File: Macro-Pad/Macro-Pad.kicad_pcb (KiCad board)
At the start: 2 copper layers, 42 x 80.5 mm, 14 parts, among them J1 USB_C_Receptacle_USB2.0_14P, U1 ESP32-S3-WROOM-1, U2 TPS62162DSG

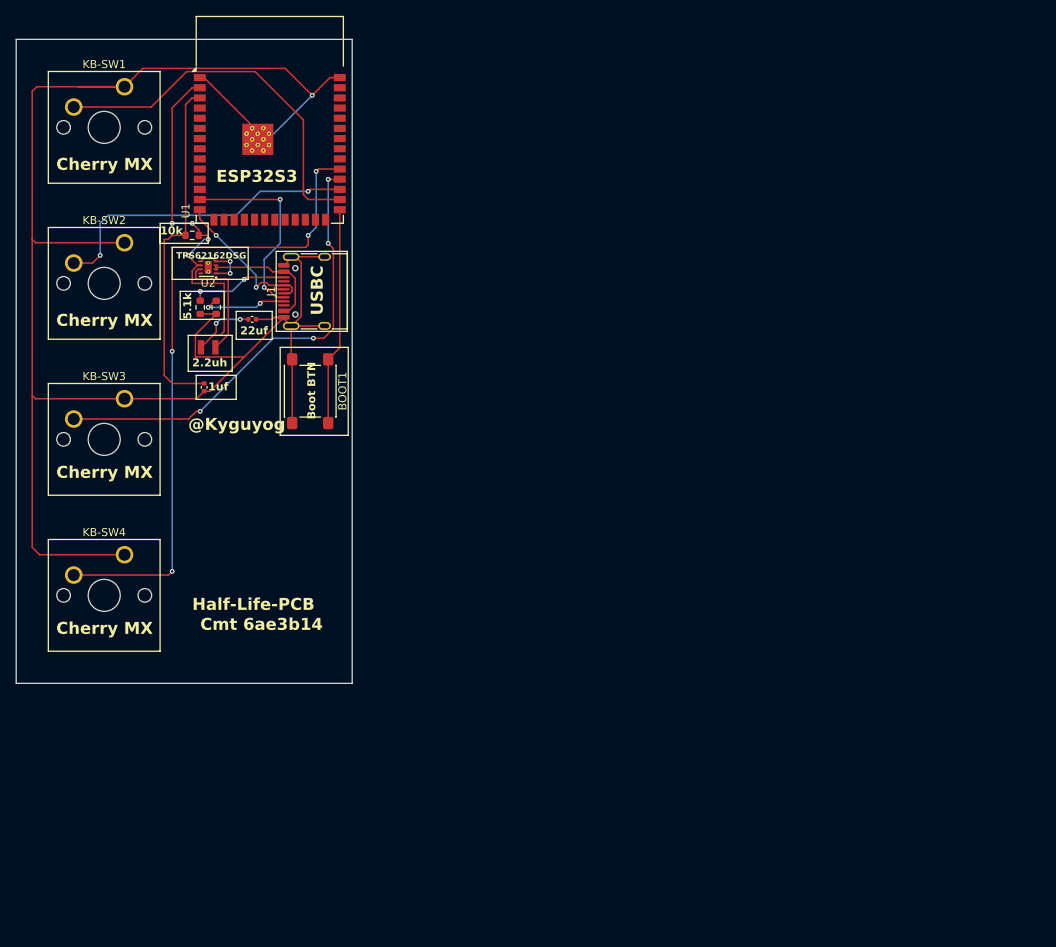
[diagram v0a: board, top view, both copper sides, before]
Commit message: re-format everything to save and optimize space
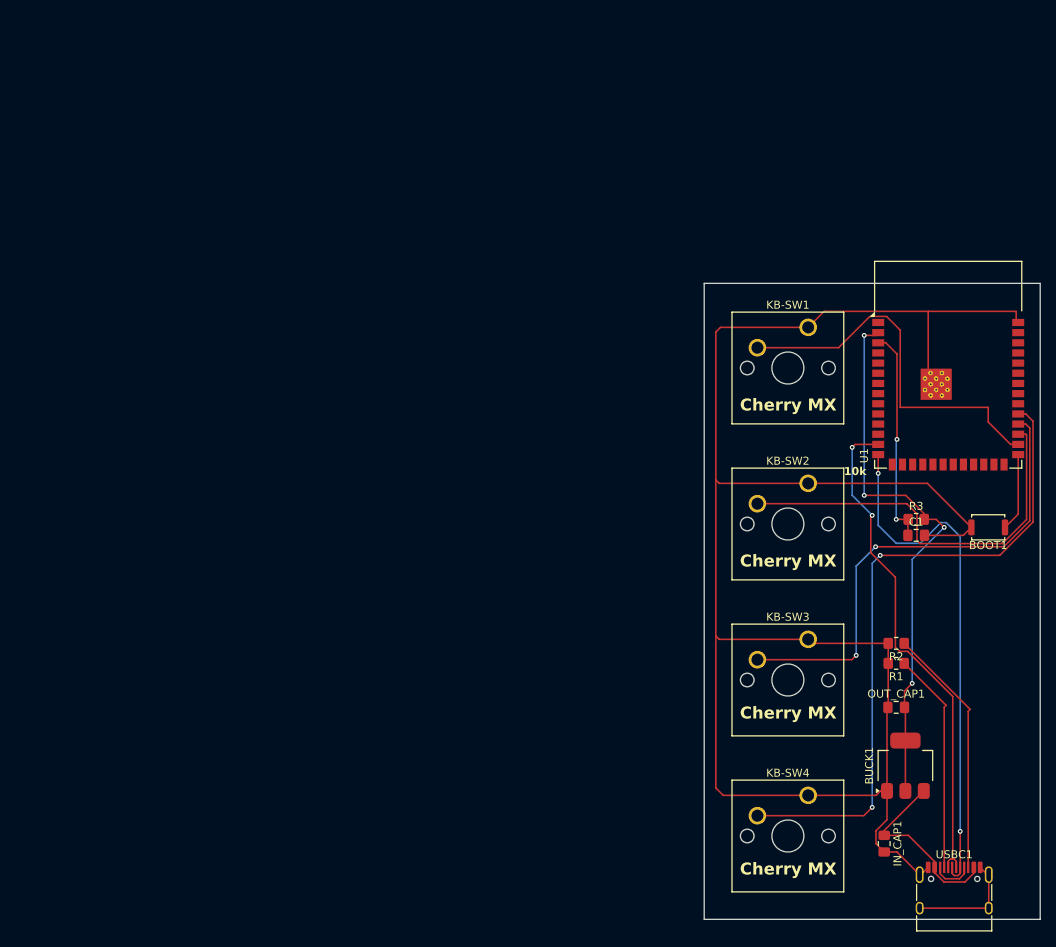
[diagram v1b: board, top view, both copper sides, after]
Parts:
- removed C2: 22uF, PCM_SparkFun-Capacitor:C_0402_1005Metric
- removed J1: USB_C_Receptacle_USB2.0_14P, Connector_USB:USB_C_Receptacle_HRO_TYPE-C-31-M-12
- removed L1: 2.2uH, PCM_SparkFun-Coil:0806
- removed U2: TPS62162DSG, Package_SON:Texas_DSG0008A_WSON-8-1EP_2x2mm_P0.5mm_EP0.9x1.6mm_ThermalVias
- added BUCK1: AMS1117-3.3, Package_TO_SOT_SMD:SOT-223-3_TabPin2, F.Cu at (124.2, 103.8)
- added IN_CAP1: 10uF, Capacitor_SMD:C_0805_2012Metric_Pad1.18x1.45mm_HandSolder, F.Cu at (121.5, 113.5)
- added OUT_CAP1: 22uF, Capacitor_SMD:C_0805_2012Metric_Pad1.18x1.45mm_HandSolder, F.Cu at (123.0, 96.5)
- added USBC1: USB_C_Receptacle_USB2.0_14P, Connector_USB:USB_C_Receptacle_HRO_TYPE-C-31-M-12, F.Cu at (130.2, 120.5)
- BOOT1: footprint Button_Switch_SMD:SW_SPST_PTS645Sx43SMTR92 -> Button_Switch_SMD:SW_Push_SPST_NO_Alps_SKRK
- C1: footprint PCM_SparkFun-Capacitor:C_0402_1005Metric -> Capacitor_SMD:C_0805_2012Metric_Pad1.18x1.45mm_HandSolder
- R1, R2, R3: footprint PCM_SparkFun-Resistor:R_0603_1608Metric -> Resistor_SMD:R_0805_2012Metric_Pad1.20x1.40mm_HandSolder
- moved R3 97.2 mm to (125.5, 73.0)
- moved R2 96.6 mm to (123.0, 88.5), turned to 180 degrees
- moved R1 95.9 mm to (123.0, 91.0), turned to 180 degrees
- moved C1 90.9 mm to (125.5, 75.0), turned to 0 degrees
- moved KB-SW1 90.6 mm to (112.0, 49.0)
- moved KB-SW2 90.6 mm to (112.0, 68.5)
- moved KB-SW3 90.6 mm to (112.0, 88.0)
- moved KB-SW4 90.6 mm to (112.0, 107.5)
- moved U1 90.2 mm to (129.5, 53.6)
- moved BOOT1 86.4 mm to (134.5, 74.0), turned to 180 degrees
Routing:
- net Net-(U1-USB_D+): track 19.2 -> 65.9 mm
- net Net-(U1-USB_D-): track 26.8 -> 63.6 mm
- net Net-(BUCK1-VI): track 0.00 -> 23.2 mm
- net Net-(USBC1-CC2): track 12.4 -> 31.5 mm, vias 2 -> 0
- net Net-(U1-IO0): track 27.3 -> 9.78 mm
- net Net-(USBC1-CC1): track 11.1 -> 27.8 mm, vias 2 -> 0
- net Net-(U1-EN): track 43.8 -> 27.3 mm, vias 0 -> 2
- net Net-(BUCK1-VO): track 52.5 -> 69.0 mm, vias 6 -> 4
- net Net-(U2-EN): track 16.1 -> 0.00 mm
- net Net-(U2-SW): track 14.9 -> 0.00 mm
- net Net-(U1-IO36): track 39.4 -> 50.6 mm, vias 2 -> 0
- net Net-(U2-AGND): track 7.29 -> 0.00 mm, vias 2 -> 0
- net (no net): track 0.00 -> 5.13 mm
- net Net-(BUCK1-GND): track 234.0 -> 238.9 mm, vias 1 -> 0
- net Net-(U1-IO37): track 57.5 -> 61.0 mm, vias 4 -> 2
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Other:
- board size 42 x 80.5 mm -> 42 x 79.5 mm
- board text removed: "1uf"
- board text removed: "2.2uh"
- board text removed: "22uf"
- board text removed: "5.1k"
- board text removed: "@Kyguyog"
- board text removed: "Boot BTN"
- board text removed: "Cmt 6ae3b14"
- board text removed: "ESP32S3"
- board text removed: "Half-Life-PCB"
- board text removed: "TPS62162DSG"
- board text removed: "USBC"
